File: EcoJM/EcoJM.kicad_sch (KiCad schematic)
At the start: 29 parts, among them J1 Screw_Terminal_01x02, J2 Screw_Terminal_01x02, J3 Conn_01x02_Pin, J4 Conn_01x02_Pin, J5 Conn_01x03_Pin, J6 Conn_01x02_Pin, J7 Conn_01x03_Pin, U1 ACS712xLCTR-30A, U2 MT2492, U3 SIT65HVD230DR, U4 AZ1117-3.3, U5 RS321BXF, U6 STM32F_dev

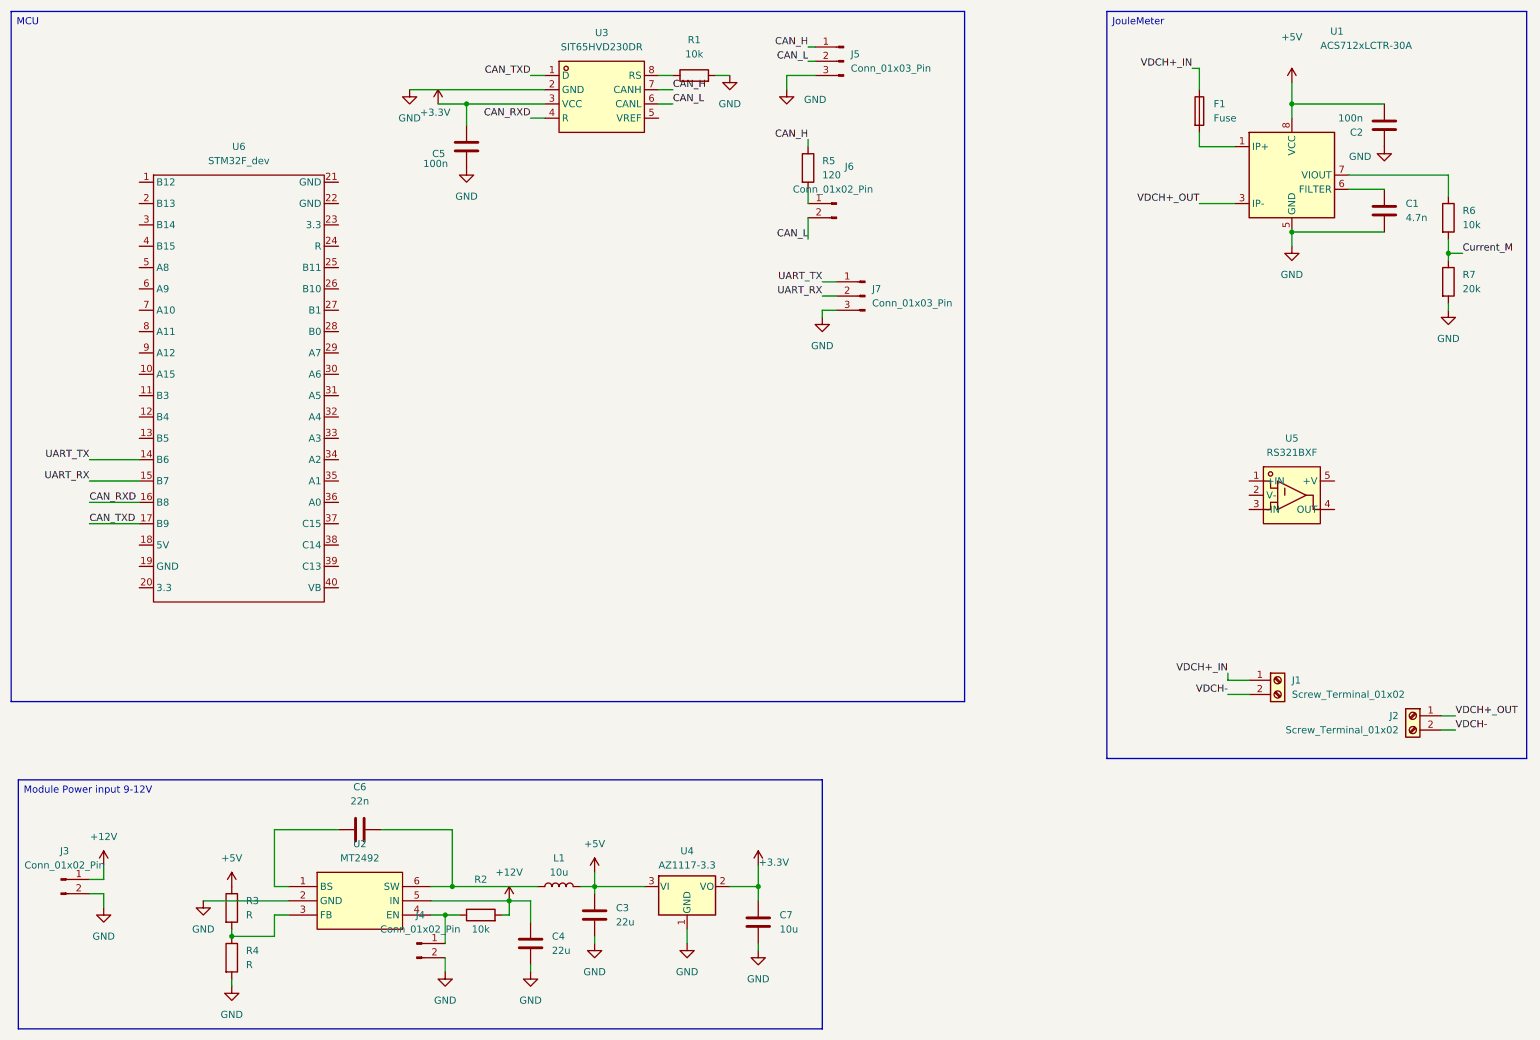
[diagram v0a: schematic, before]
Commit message: Schematic = 100% , Footprints=100%
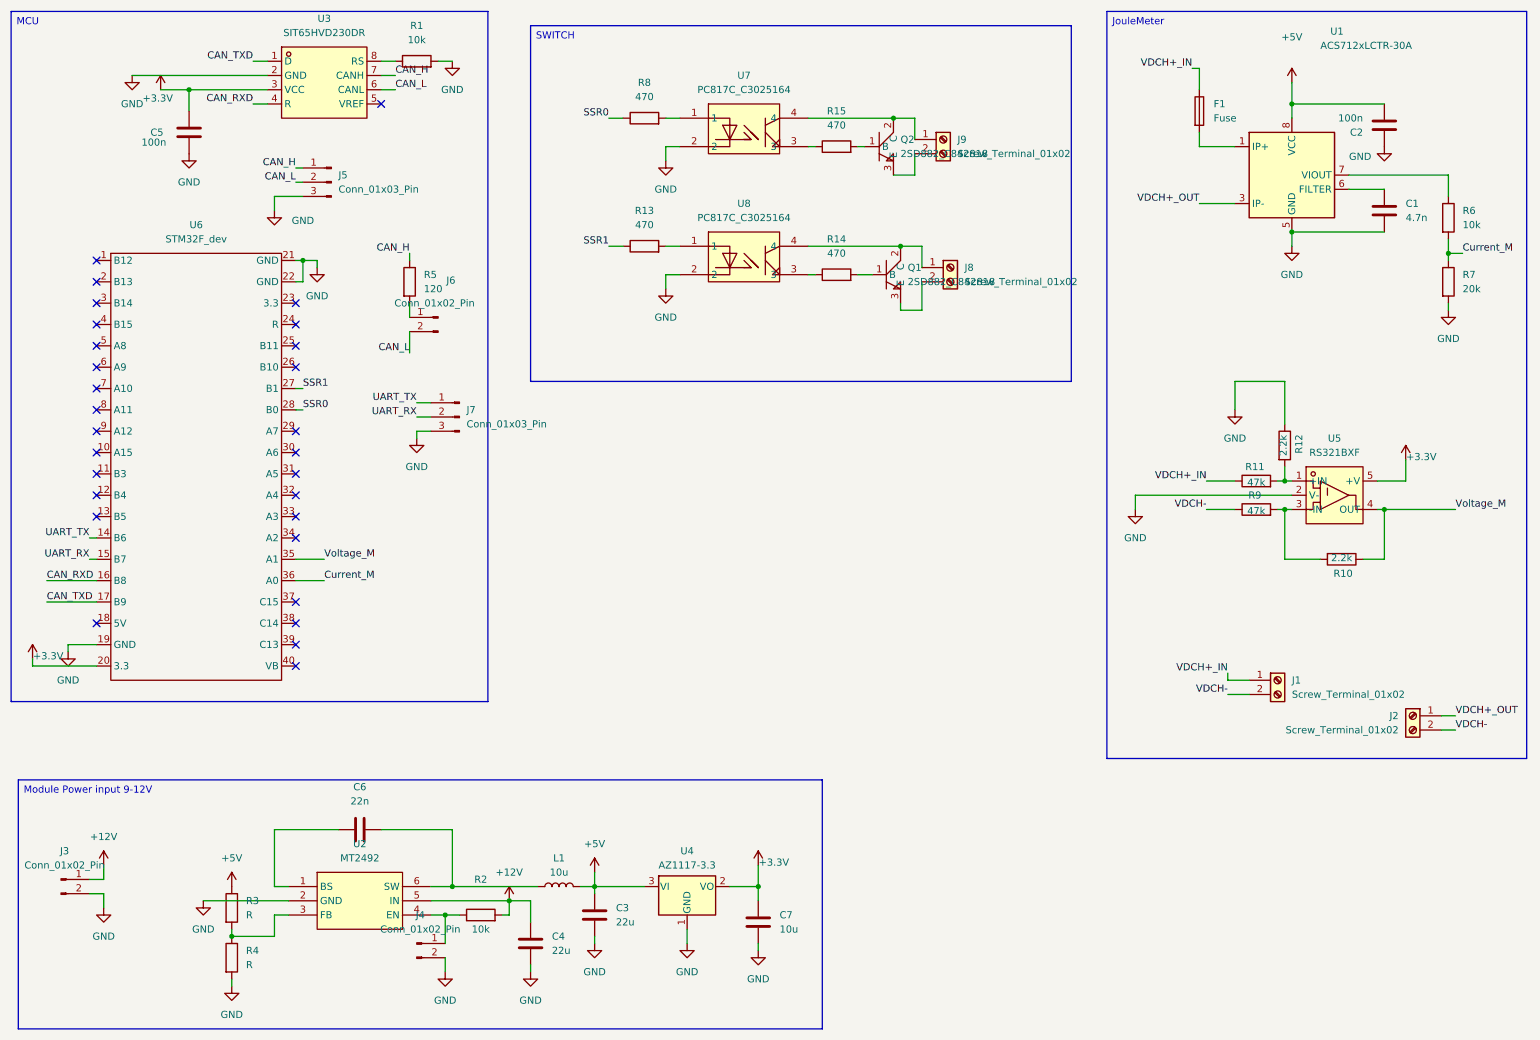
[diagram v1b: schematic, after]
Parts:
- added J8, J9: Screw_Terminal_01x02, TerminalBlock_Phoenix:TerminalBlock_Phoenix_PT-1,5-2-3.5-H_1x02_P3.50mm_Horizontal, symbol Connector:Screw_Terminal_01x02
- added Q1, Q2: 2SD882_C842818, EasyEDA:SOT-89-3_L4.5-W2.5-P1.50-LS4.1-BR, symbol EasyEDA:2SD882_C842818
- added R10, R12: 2.2k, Resistor_SMD:R_1206_3216Metric_Pad1.30x1.75mm_HandSolder, symbol Device:R
- added R11, R9: 47k, Resistor_SMD:R_1206_3216Metric_Pad1.30x1.75mm_HandSolder, symbol Device:R
- added R13, R14, R15, R8: 470, Resistor_SMD:R_1206_3216Metric_Pad1.30x1.75mm_HandSolder, symbol Device:R
- added U7, U8: PC817C_C3025164, EasyEDA:OPTO-SMD-4_L4.6-W6.5-P2.54-LS10.3-TL, symbol EasyEDA:PC817C_C3025164
- C1, C2, C3, C4, C5, C6, C7: footprint (none) -> LED_SMD:LED_1206_3216Metric_Pad1.42x1.75mm_HandSolder
- J3: footprint (none) -> Connector_JST:JST_XH_B2B-XH-A_1x02_P2.50mm_Vertical
- J4, J6: footprint (none) -> Connector_PinHeader_2.54mm:PinHeader_1x02_P2.54mm_Vertical
- J5, J7: footprint (none) -> Connector_JST:JST_XH_B3B-XH-A_1x03_P2.50mm_Vertical
- L1: footprint (none) -> EasyEDA:IND-SMD_L7.2-W6.6_GPSR07X0
- R1, R2, R3, R4, R5, R6, R7: footprint (none) -> Resistor_SMD:R_1206_3216Metric_Pad1.30x1.75mm_HandSolder
- U6: footprint (none) -> dev_board:STM32F_devboard
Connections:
- net +3.3V: now also U5.5 (+V), U6.20 (3.3)
- net Current_M: now also U6.36 (A0)
- net GND: now also U5.2 (V-), U6.19 (GND), U6.21 (GND), U6.22 (GND), R12.1, U7.2, U8.2
- net VDCH+_IN: now also R11.1
- net VDCH-: now also R9.1
- net at U5.1 (+IN): now also R11.2, R12.2
- net at U5.3 (-IN): now also R10.2, R9.2
- net Voltage_M: now reaches U5.4 (OUT)
- net Voltage_M: now also U6.35 (A1), R10.1
- net SSR1: now reaches U6.27 (B1)
- net SSR1: now also R13.1
- net SSR0: now reaches U6.28 (B0)
- net SSR0: now also R8.1
- new net: R13.2, U8.1
- new net: R14.1, U8.3
- new net: J8.1 (Pin_1), Q1.2 (C), U8.4
- new net: J9.1 (Pin_1), Q2.2 (C), U7.4
- new net: J9.2 (Pin_2), Q2.3 (E)
- new net: Q1.1 (B), R14.2
- new net: R8.2, U7.1
- new net: R15.1, U7.3
- new net: Q2.1 (B), R15.2
- new net: J8.2 (Pin_2), Q1.3 (E)
- no-connect marks 0 -> 29
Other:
- moved on the sheet: C5, J5, J6, J7, R1, R5, U3, U5, U6
